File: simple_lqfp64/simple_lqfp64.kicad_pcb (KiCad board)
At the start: 2 copper layers, 52 parts, among them P1 CONN_01X02, P10 CONN_01X04, P11 CONN_01X03, P12 CONN_01X03, P13 USB_A, P14 CONN_01X01, P15 CONN_01X01, P16 CONN_01X01, P17 CONN_01X01, P18 CONN_01X01, P19 CONN_01X01, P2 CONN_01X03, P20 CONN_01X01, P21 CONN_01X01, P22 CONN_01X01, P23 CONN_01X01, P24 CONN_01X01, P25 CONN_01X01, P26 CONN_01X01, P27 CONN_01X01, P28 CONN_01X01, P29 CONN_01X01, P3 CONN_01X04, P30 CONN_01X01, P31 CONN_01X01, P32 CONN_01X01, P33 CONN_01X01, P34 CONN_02X03, P4 CONN_01X04, P5 CONN_01X01, P6 CONN_01X04, P7 CONN_01X03, P8 CONN_01X06, P9 CONN_01X07, SW1 SW_PUSH, U1 STM32F103RCTx, U2 AP1117D33, Y1 Crystal, Y2 Crystal

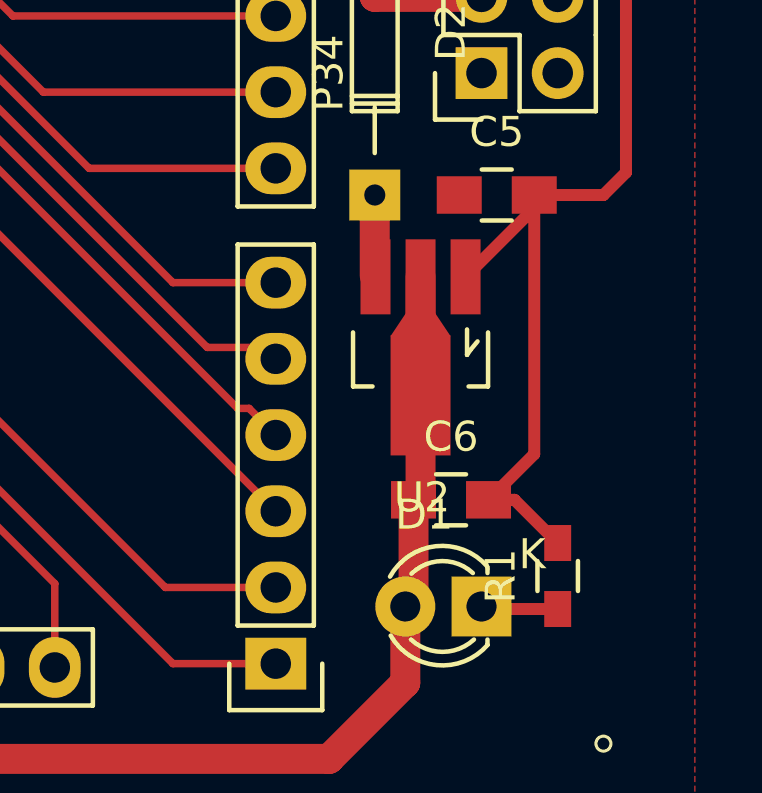
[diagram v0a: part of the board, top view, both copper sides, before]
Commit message: charger libs
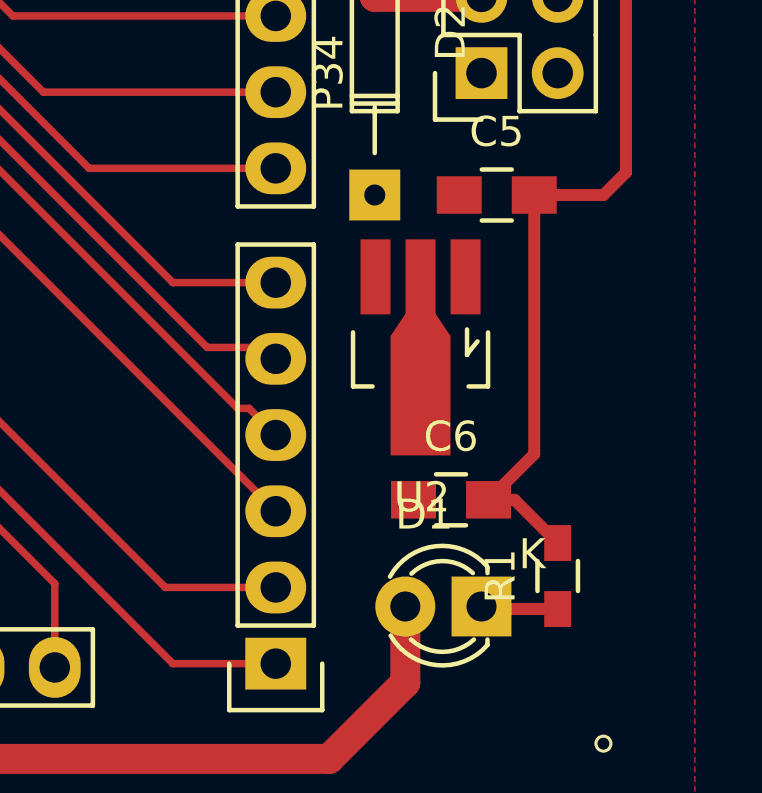
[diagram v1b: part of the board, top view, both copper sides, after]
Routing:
- net +3V3: track 207.0 -> 196.5 mm
- net GND: track 292.8 -> 289.6 mm
- net Net-(C5-Pad1): track 2.74 -> 0.04 mm
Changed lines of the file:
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@@
   (general
     (links 116)
-    (no_connects 1)
+    (no_connects 5)
     (area 109.856001 36.266 193.670001 105.062001)
     (thickness 1.6)
     (drawings 7)
-    (tracks 397)
+    (tracks 393)
     (zones 0)
     (modules 52)
@@
   )
   (setup
-    (last_trace_width 1)
+    (last_trace_width 0.25)
     (user_trace_width 0.4)
     (user_trace_width 0.5)
@@
   (segment (start 136.017 62.865) (end 132.969 65.913) (width 0.25) (layer F.Cu) (net 1))
   (segment (start 136.037 61.67406) (end 136.017 61.69406) (width 0.25) (layer F.Cu) (net 1))
-  (segment (start 186.162 92.964) (end 187.028 92.964) (width 0.4) (layer F.Cu) (net 2) (status 400000))
-  (segment (start 187.028 92.964) (end 188.468 94.404) (width 0.4) (layer F.Cu) (net 2) (status 800000))
-  (segment (start 187.686 82.804) (end 187.686 91.44) (width 0.4) (layer F.Cu) (net 2) (status 400000))
-  (segment (start 187.686 91.44) (end 186.162 92.964) (width 0.4) (layer F.Cu) (net 2) (status 800000))
-  (segment (start 187.686 82.804) (end 187.686 83.2431) (width 0.4) (layer F.Cu) (net 2) (status C00000))
-  (segment (start 187.686 83.2431) (end 185.39714 85.53196) (width 0.4) (layer F.Cu) (net 2) (status C00000))
-  (segment (start 190.74384 65.41008) (end 190.74384 82.05216) (width 0.4) (layer F.Cu) (net 2) (status 400000))
-  (segment (start 189.992 82.804) (end 187.686 82.804) (width 0.4) (layer F.Cu) (net 2) (status 800000))
+  (segment (start 186.162 92.964) (end 187.028 92.964) (width 0.4) (layer F.Cu) (net 2))
+  (segment (start 187.028 92.964) (end 188.468 94.404) (width 0.4) (layer F.Cu) (net 2))
+  (segment (start 187.686 82.804) (end 187.686 91.44) (width 0.4) (layer F.Cu) (net 2))
+  (segment (start 187.686 91.44) (end 186.162 92.964) (width 0.4) (layer F.Cu) (net 2))
+  (segment (start 187.686 82.804) (end 187.686 83.2431) (width 0.4) (layer F.Cu) (net 2))
+  (segment (start 190.74384 65.41008) (end 190.74384 82.05216) (width 0.4) (layer F.Cu) (net 2))
+  (segment (start 189.992 82.804) (end 187.686 82.804) (width 0.4) (layer F.Cu) (net 2))
   (segment (start 190.74384 82.05216) (end 189.992 82.804) (width 0.4) (layer F.Cu) (net 2))
   (segment (start 128.651 76.22) (end 128.651 73.8505) (width 0.25) (layer F.Cu) (net 2))
@@
   (segment (start 160.528 84.582) (end 156.718 84.582) (width 0.25) (layer F.Cu) (net 47))
   (segment (start 171.704 95.758) (end 160.528 84.582) (width 0.25) (layer F.Cu) (net 47))
-  (segment (start 185.928 76.2) (end 182.372 76.2) (width 1) (layer F.Cu) (net 48) (status 400000))
-  (segment (start 182.36946 76.19746) (end 182.36946 72.64348) (width 1) (layer F.Cu) (net 48) (status 800000))
+  (segment (start 185.928 76.2) (end 182.372 76.2) (width 1) (layer F.Cu) (net 48))
+  (segment (start 182.36946 76.19746) (end 182.36946 72.64348) (width 1) (layer F.Cu) (net 48))
   (segment (start 182.372 76.2) (end 182.36946 76.19746) (width 0.4) (layer F.Cu) (net 48))
   (segment (start 185.14568 61.7601) (end 176.9999 61.7601) (width 0.25) (layer F.Cu) (net 49))
@@
   (segment (start 164.81 72.68) (end 160.64 72.68) (width 0.25) (layer F.Cu) (net 50))
   (segment (start 176.53 60.96) (end 164.81 72.68) (width 0.25) (layer F.Cu) (net 50))
-  (segment (start 183.388 96.52) (end 183.388 99.06) (width 1) (layer F.Cu) (net 52) (status 400000))
+  (segment (start 183.388 96.52) (end 183.388 99.06) (width 1) (layer F.Cu) (net 52))
   (segment (start 180.848 101.6) (end 147.066 101.6) (width 1) (layer F.Cu) (net 52))
   (segment (start 183.388 99.06) (end 180.848 101.6) (width 1) (layer F.Cu) (net 52))
-  (segment (start 183.662 92.964) (end 183.662 96.246) (width 1) (layer F.Cu) (net 52) (status C00000))
-  (segment (start 183.662 96.246) (end 183.388 96.52) (width 0.4) (layer F.Cu) (net 52) (status C00000))
-  (segment (start 183.896 85.53196) (end 183.896 87.1347) (width 0.4) (layer F.Cu) (net 52) (status C00000))
-  (segment (start 183.896 87.1347) (end 183.896 89.4842) (width 0.4) (layer F.Cu) (net 52) (status C00000))
-  (segment (start 183.896 85.53196) (end 183.896 92.73) (width 1) (layer F.Cu) (net 52) (status C00000))
-  (segment (start 183.896 92.73) (end 183.662 92.964) (width 0.4) (layer F.Cu) (net 52) (status C00000))
+  (segment (start 183.662 96.246) (end 183.388 96.52) (width 0.4) (layer F.Cu) (net 52))
+  (segment (start 183.896 85.53196) (end 183.896 87.1347) (width 0.4) (layer F.Cu) (net 52))
+  (segment (start 183.896 87.1347) (end 183.896 89.4842) (width 0.4) (layer F.Cu) (net 52))
+  (segment (start 183.896 92.73) (end 183.662 92.964) (width 0.4) (layer F.Cu) (net 52))
   (segment (start 156.2735 73.3425) (end 156.5275 73.3425) (width 0.25) (layer F.Cu) (net 52))
   (segment (start 158.6865 71.1835) (end 160.6365 71.1835) (width 0.25) (layer F.Cu) (net 52))
@@
   (segment (start 180.086 52.832) (end 175.088 52.832) (width 0.25) (layer F.Cu) (net 56))
   (segment (start 175.088 52.832) (end 158.69 69.23) (width 0.25) (layer F.Cu) (net 56))
-  (segment (start 188.468 96.604) (end 186.012 96.604) (width 0.4) (layer F.Cu) (net 57) (status C00000))
-  (segment (start 186.012 96.604) (end 185.928 96.52) (width 0.4) (layer F.Cu) (net 57) (status C00000))
+  (segment (start 188.468 96.604) (end 186.012 96.604) (width 0.4) (layer F.Cu) (net 57))
+  (segment (start 186.012 96.604) (end 185.928 96.52) (width 0.4) (layer F.Cu) (net 57))
   (segment (start 130.683 78.74) (end 128.671 78.74) (width 0.25) (layer F.Cu) (net 58))
   (segment (start 128.671 78.74) (end 128.651 78.72) (width 0.25) (layer F.Cu) (net 58))
@@
   (segment (start 145.022 74.18) (end 149.24 74.18) (width 0.25) (layer F.Cu) (net 58))
   (segment (start 140.462 78.74) (end 145.022 74.18) (width 0.25) (layer F.Cu) (net 58))
-  (segment (start 182.36946 82.80348) (end 182.36946 85.50656) (width 1) (layer F.Cu) (net 59) (status C00000))
-  (segment (start 182.36946 85.50656) (end 182.39486 85.53196) (width 0.4) (layer F.Cu) (net 59) (status C00000))
-  (segment (start 185.42 72.644) (end 185.42 73.152) (width 1) (layer F.Cu) (net 60) (status 800000))
-  (segment (start 185.42 73.152) (end 185.928 73.66) (width 1) (layer F.Cu) (net 60) (status C00000))
-  (segment (start 185.42 69.342) (end 185.42 72.644) (width 1) (layer F.Cu) (net 60) (status 400000))
-  (segment (start 185.42 73.152) (end 185.928 73.66) (width 0.4) (layer F.Cu) (net 60) (status C00000))
-  (segment (start 185.14568 62.5602) (end 182.4482 62.5602) (width 0.4) (layer F.Cu) (net 60) (status 400000))
-  (segment (start 182.626 69.342) (end 185.42 69.342) (width 1) (layer F.Cu) (net 60) (status 800000))
+  (segment (start 182.36946 85.50656) (end 182.39486 85.53196) (width 0.4) (layer F.Cu) (net 59))
+  (segment (start 185.42 72.644) (end 185.42 73.152) (width 1) (layer F.Cu) (net 60))
+  (segment (start 185.42 73.152) (end 185.928 73.66) (width 1) (layer F.Cu) (net 60))
+  (segment (start 185.42 69.342) (end 185.42 72.644) (width 1) (layer F.Cu) (net 60))
+  (segment (start 185.42 73.152) (end 185.928 73.66) (width 0.4) (layer F.Cu) (net 60))
+  (segment (start 185.14568 62.5602) (end 182.4482 62.5602) (width 0.4) (layer F.Cu) (net 60))
+  (segment (start 182.626 69.342) (end 185.42 69.342) (width 1) (layer F.Cu) (net 60))
   (segment (start 182.372 69.088) (end 182.626 69.342) (width 1) (layer F.Cu) (net 60))
   (segment (start 182.372 62.6364) (end 182.372 69.088) (width 1) (layer F.Cu) (net 60))
@@
     (connect_pads (clearance 0.8))
     (min_thickness 0.4)
-    (fill yes (arc_segments 16) (thermal_gap 0.508) (thermal_bridge_width 0.508))
+    (fill (arc_segments 16) (thermal_gap 0.508) (thermal_bridge_width 0.508))
     (polygon
       (pts
